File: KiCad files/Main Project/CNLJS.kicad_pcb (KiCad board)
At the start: 2 copper layers, 150 x 150 mm, 169 parts, among them J1 USBasp, J17 Conn_01x03_Male, J18 Conn_01x03_Male, J19 Conn_01x03_Male, J2 USB_C_Receptacle_USB2.0, J20 Conn_01x03_Male, Q1 Si2319CDS, SW1 SW_Push, SW2 SW_SPDT, U17 PCF8575, U18 ATmega328-A, U2 MCP73871-2CC, U3 CH340C, U4 2108, Y1 16MHz

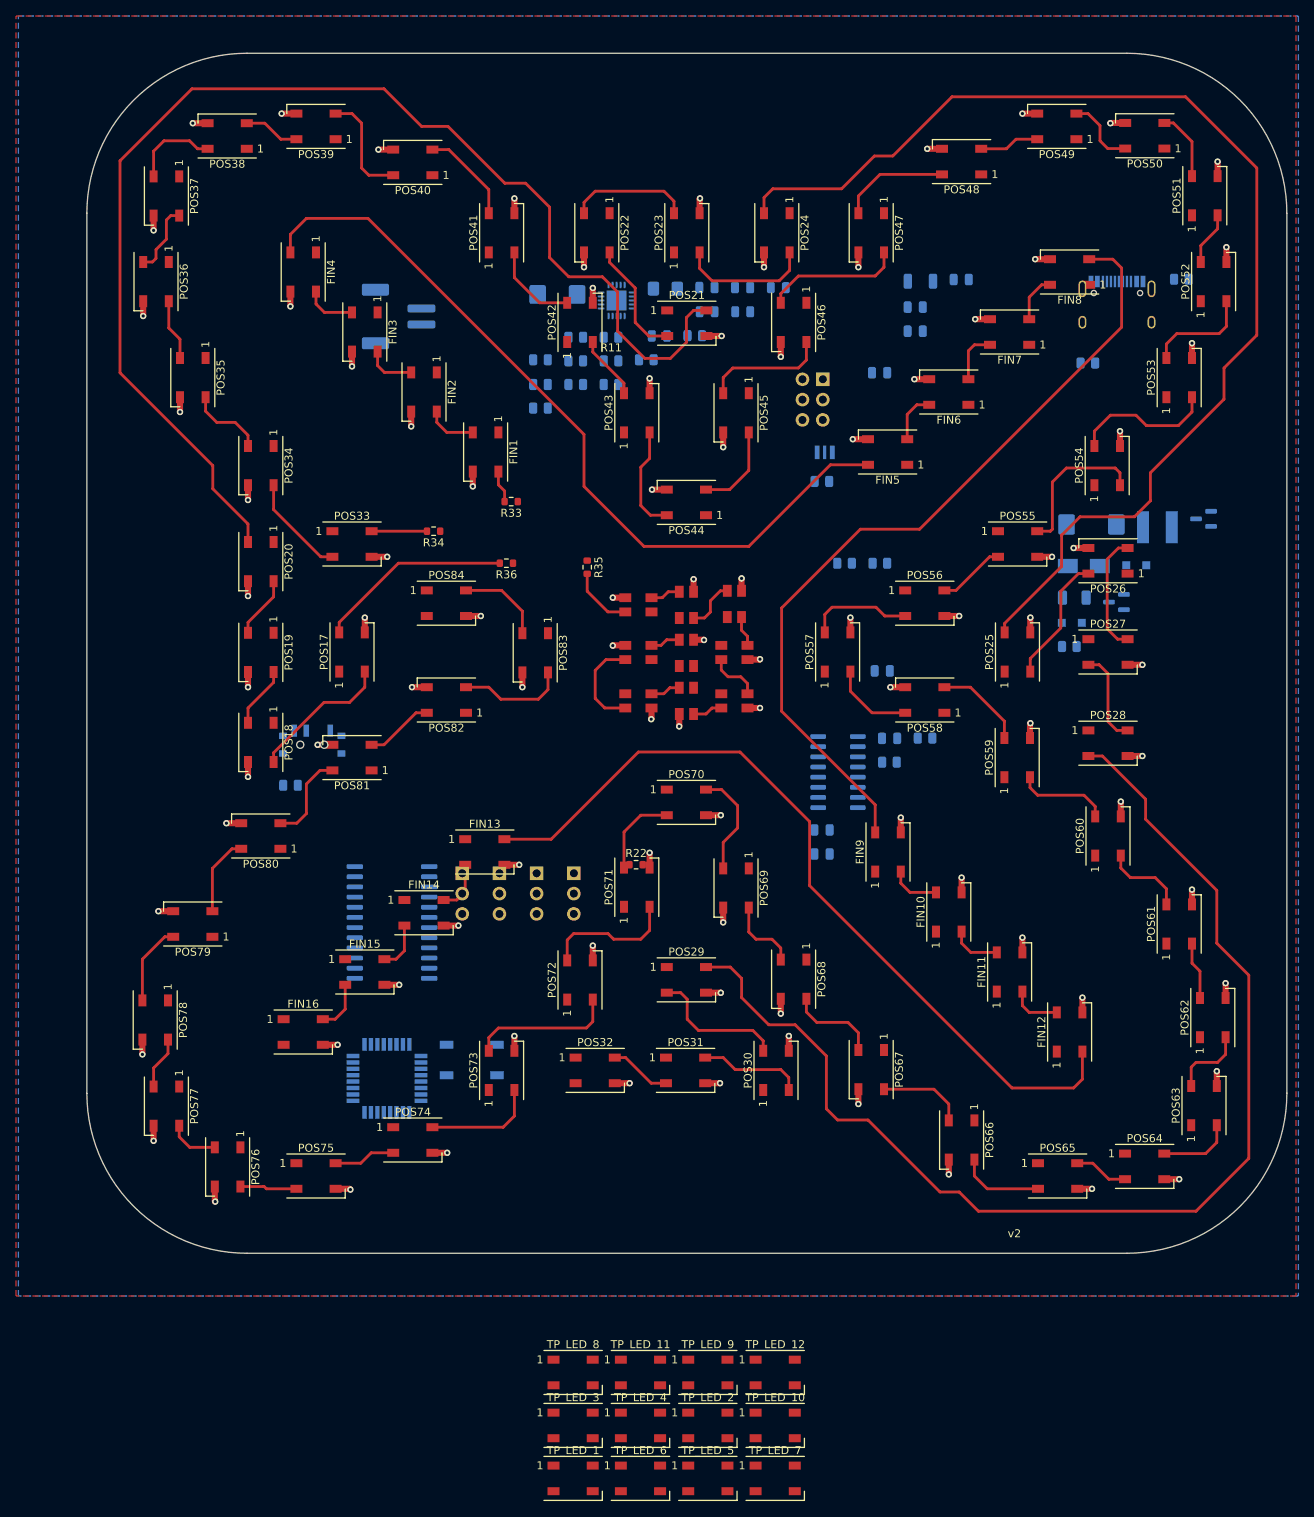
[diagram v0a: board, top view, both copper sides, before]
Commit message: Update CNLJS.kicad_pcb
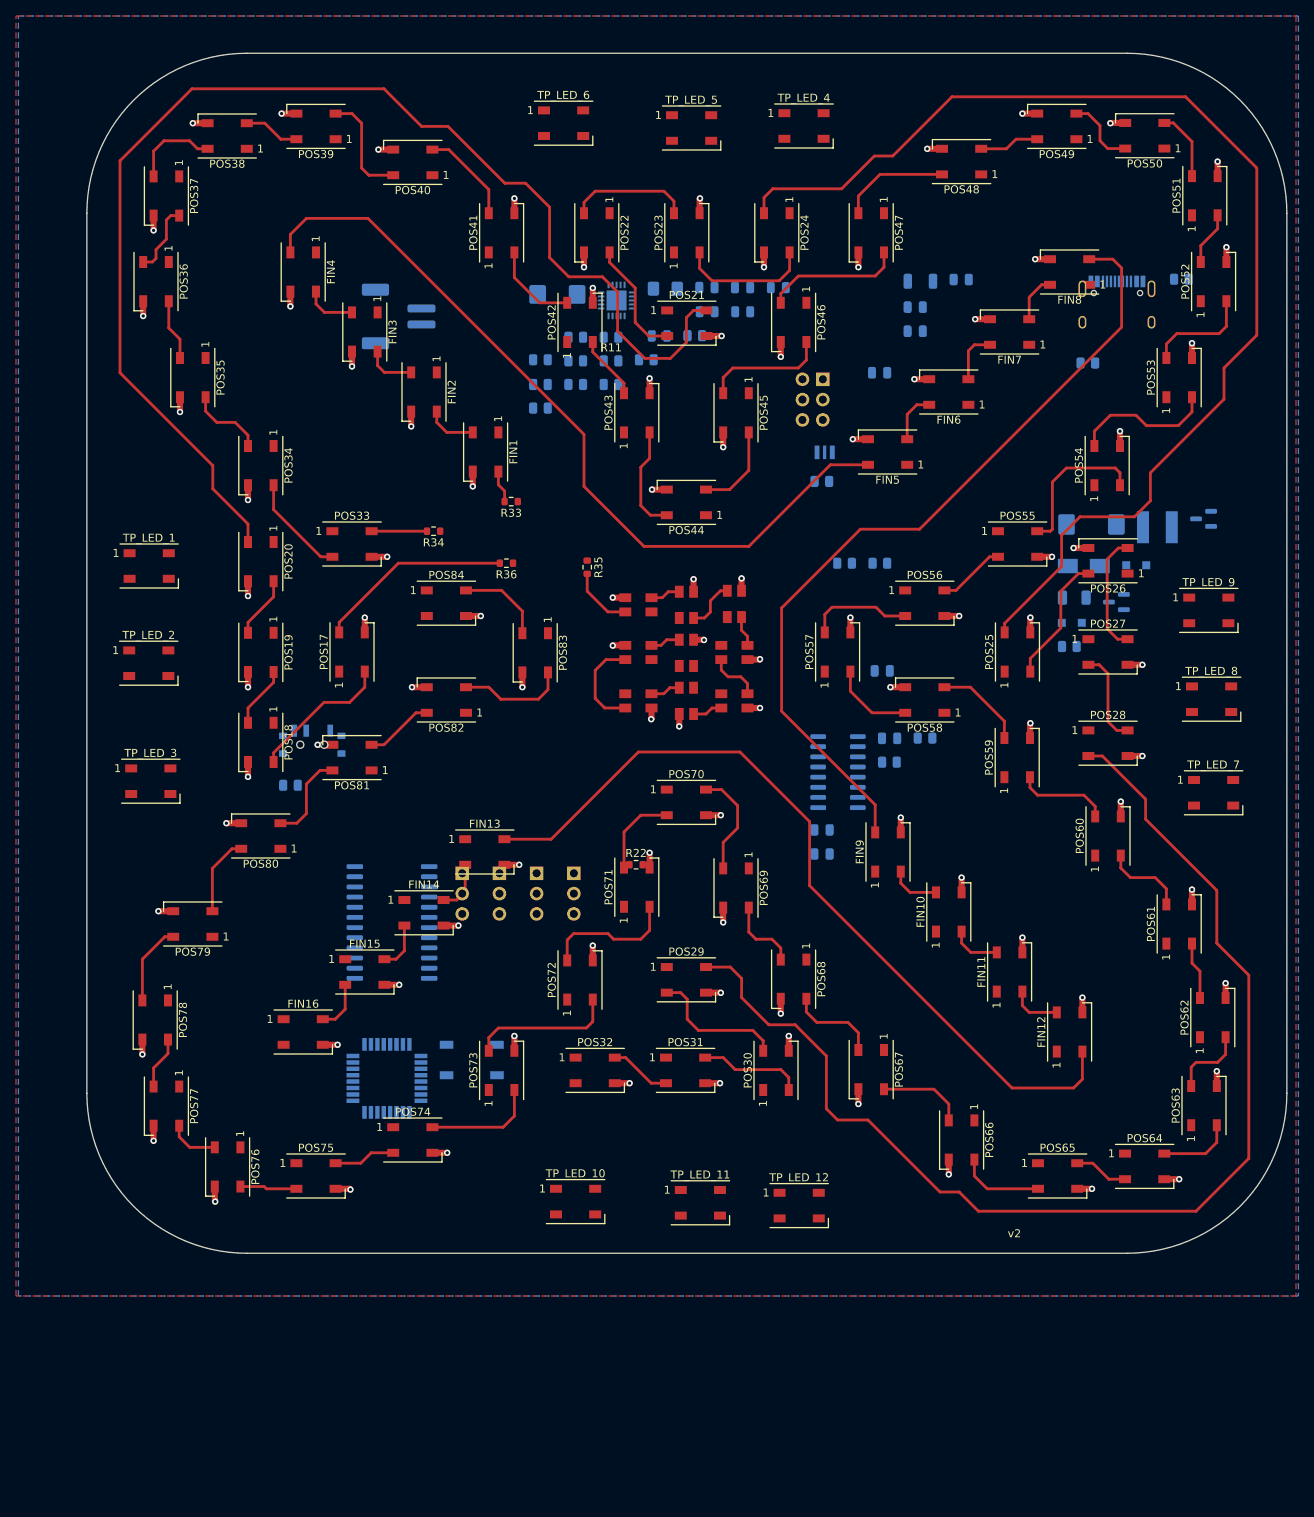
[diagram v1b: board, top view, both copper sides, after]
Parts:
- moved TP_LED_6 169.7 mm to (127.3, 26.8)
- moved TP_LED_5 168.8 mm to (143.3, 27.4)
- moved TP_LED_4 163.7 mm to (157.3, 27.1)
- moved TP_LED_1 125.8 mm to (75.5, 82.1)
- moved TP_LED_2 118.2 mm to (75.5, 94.2)
- moved TP_LED_8 116.0 mm to (208.3, 98.8)
- moved TP_LED_9 114.0 mm to (207.9, 87.7)
- moved TP_LED_7 101.7 mm to (208.6, 110.5)
- moved TP_LED_3 96.3 mm to (75.7, 109.0)
- moved TP_LED_10 37.5 mm to (128.8, 161.6)
- moved TP_LED_11 22.5 mm to (144.4, 161.7)
- moved TP_LED_12 21.1 mm to (156.8, 162.1)
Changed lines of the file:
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@@
   )
   (footprint "LED_SMD:LED_WS2812B_PLCC4_5.0x5.0mm_P3.2mm" (layer "F.Cu")
-    (at 145.33 182.91)
+    (at 207.95 87.65)
     (descr "https://cdn-shop.adafruit.com/datasheets/WS2812B.pdf")
     (tags "LED RGB NeoPixel")
@@
   )
   (footprint "LED_SMD:LED_WS2812B_PLCC4_5.0x5.0mm_P3.2mm" (layer "F.Cu")
-    (at 145.33 189.53)
+    (at 75.45 94.25)
     (descr "https://cdn-shop.adafruit.com/datasheets/WS2812B.pdf")
     (tags "LED RGB NeoPixel")
@@
   )
   (footprint "LED_SMD:LED_WS2812B_PLCC4_5.0x5.0mm_P3.2mm" (layer "F.Cu")
-    (at 136.91 189.53)
+    (at 157.35 27.1)
     (descr "https://cdn-shop.adafruit.com/datasheets/WS2812B.pdf")
     (tags "LED RGB NeoPixel")
@@
   )
   (footprint "LED_SMD:LED_WS2812B_PLCC4_5.0x5.0mm_P3.2mm" (layer "F.Cu")
-    (at 153.75 182.91)
+    (at 156.75 162.05)
     (descr "https://cdn-shop.adafruit.com/datasheets/WS2812B.pdf")
     (tags "LED RGB NeoPixel")
@@
   )
   (footprint "LED_SMD:LED_WS2812B_PLCC4_5.0x5.0mm_P3.2mm" (layer "F.Cu")
-    (at 128.49 182.91)
+    (at 208.3 98.75)
     (descr "https://cdn-shop.adafruit.com/datasheets/WS2812B.pdf")
     (tags "LED RGB NeoPixel")
@@
   )
   (footprint "LED_SMD:LED_WS2812B_PLCC4_5.0x5.0mm_P3.2mm" (layer "F.Cu")
-    (at 136.91 182.91)
+    (at 144.4 161.7)
     (descr "https://cdn-shop.adafruit.com/datasheets/WS2812B.pdf")
     (tags "LED RGB NeoPixel")
@@
   )
   (footprint "LED_SMD:LED_WS2812B_PLCC4_5.0x5.0mm_P3.2mm" (layer "F.Cu")
-    (at 128.49 196.15)
+    (at 75.5 82.1)
     (descr "https://cdn-shop.adafruit.com/datasheets/WS2812B.pdf")
     (tags "LED RGB NeoPixel")
@@
   )
   (footprint "LED_SMD:LED_WS2812B_PLCC4_5.0x5.0mm_P3.2mm" (layer "F.Cu")
-    (at 145.33 196.15)
+    (at 143.3 27.35)
     (descr "https://cdn-shop.adafruit.com/datasheets/WS2812B.pdf")
     (tags "LED RGB NeoPixel")
@@
   )
   (footprint "LED_SMD:LED_WS2812B_PLCC4_5.0x5.0mm_P3.2mm" (layer "F.Cu")
-    (at 153.75 189.53)
+    (at 128.8 161.55)
     (descr "https://cdn-shop.adafruit.com/datasheets/WS2812B.pdf")
     (tags "LED RGB NeoPixel")
@@
   )
   (footprint "LED_SMD:LED_WS2812B_PLCC4_5.0x5.0mm_P3.2mm" (layer "F.Cu")
-    (at 128.49 189.53)
+    (at 75.7 109)
     (descr "https://cdn-shop.adafruit.com/datasheets/WS2812B.pdf")
     (tags "LED RGB NeoPixel")
@@
   )
   (footprint "LED_SMD:LED_WS2812B_PLCC4_5.0x5.0mm_P3.2mm" (layer "F.Cu")
-    (at 153.75 196.15)
+    (at 208.55 110.45)
     (descr "https://cdn-shop.adafruit.com/datasheets/WS2812B.pdf")
     (tags "LED RGB NeoPixel")
@@
   )
   (footprint "LED_SMD:LED_WS2812B_PLCC4_5.0x5.0mm_P3.2mm" (layer "F.Cu")
-    (at 136.91 196.15)
+    (at 127.3 26.75)
     (descr "https://cdn-shop.adafruit.com/datasheets/WS2812B.pdf")
     (tags "LED RGB NeoPixel")
